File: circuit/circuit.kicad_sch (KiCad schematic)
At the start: 23 parts, among them SW101 SW_Push, SW102 SW_Push, SW103 SW_Push, SW104 SW_Push, SW105 SW_Push, SW106 SW_Push, SW107 SW_Push, SW108 SW_Push, SW109 SW_Push, SW110 SW_Push, U5 ESP32-S3-DevKitC

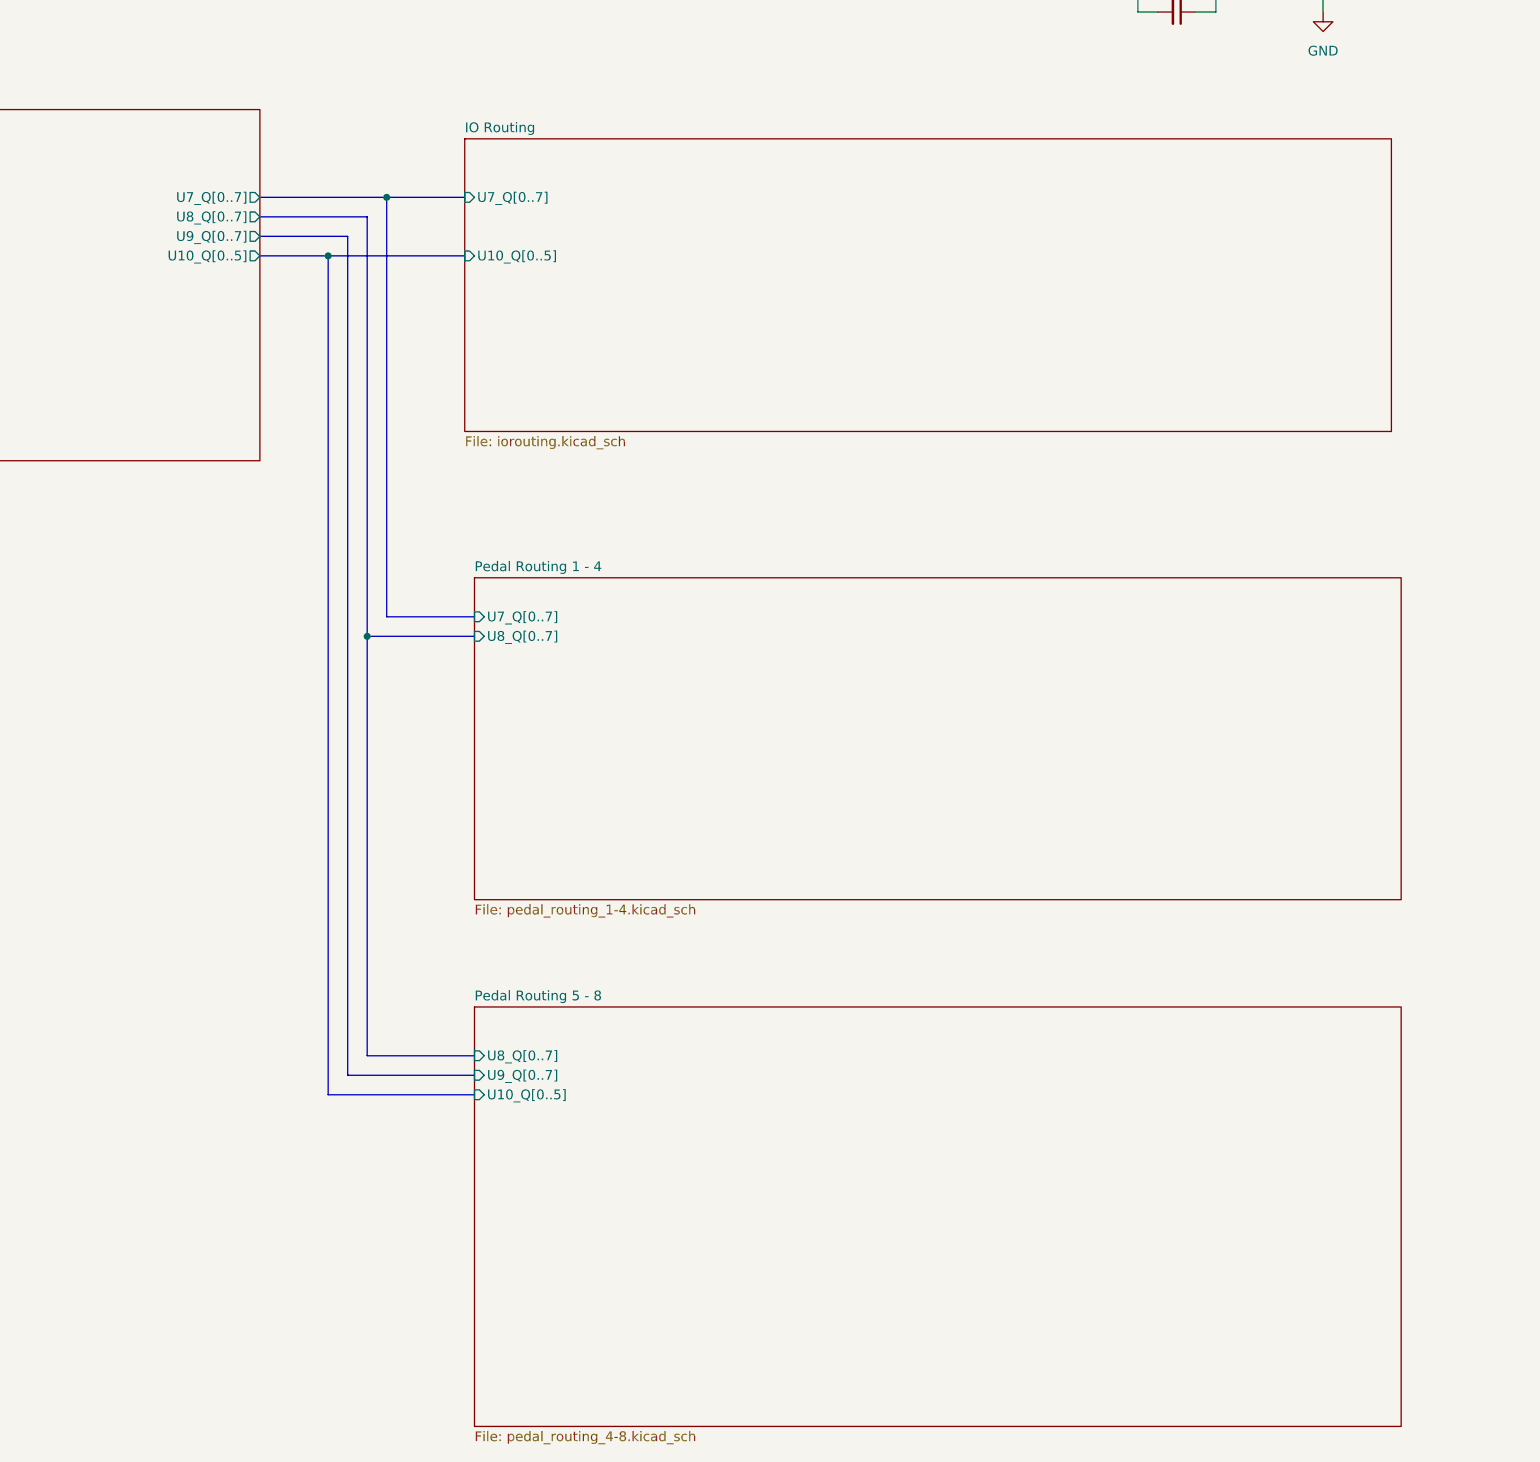
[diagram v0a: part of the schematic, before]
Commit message: Hopefully close to finished
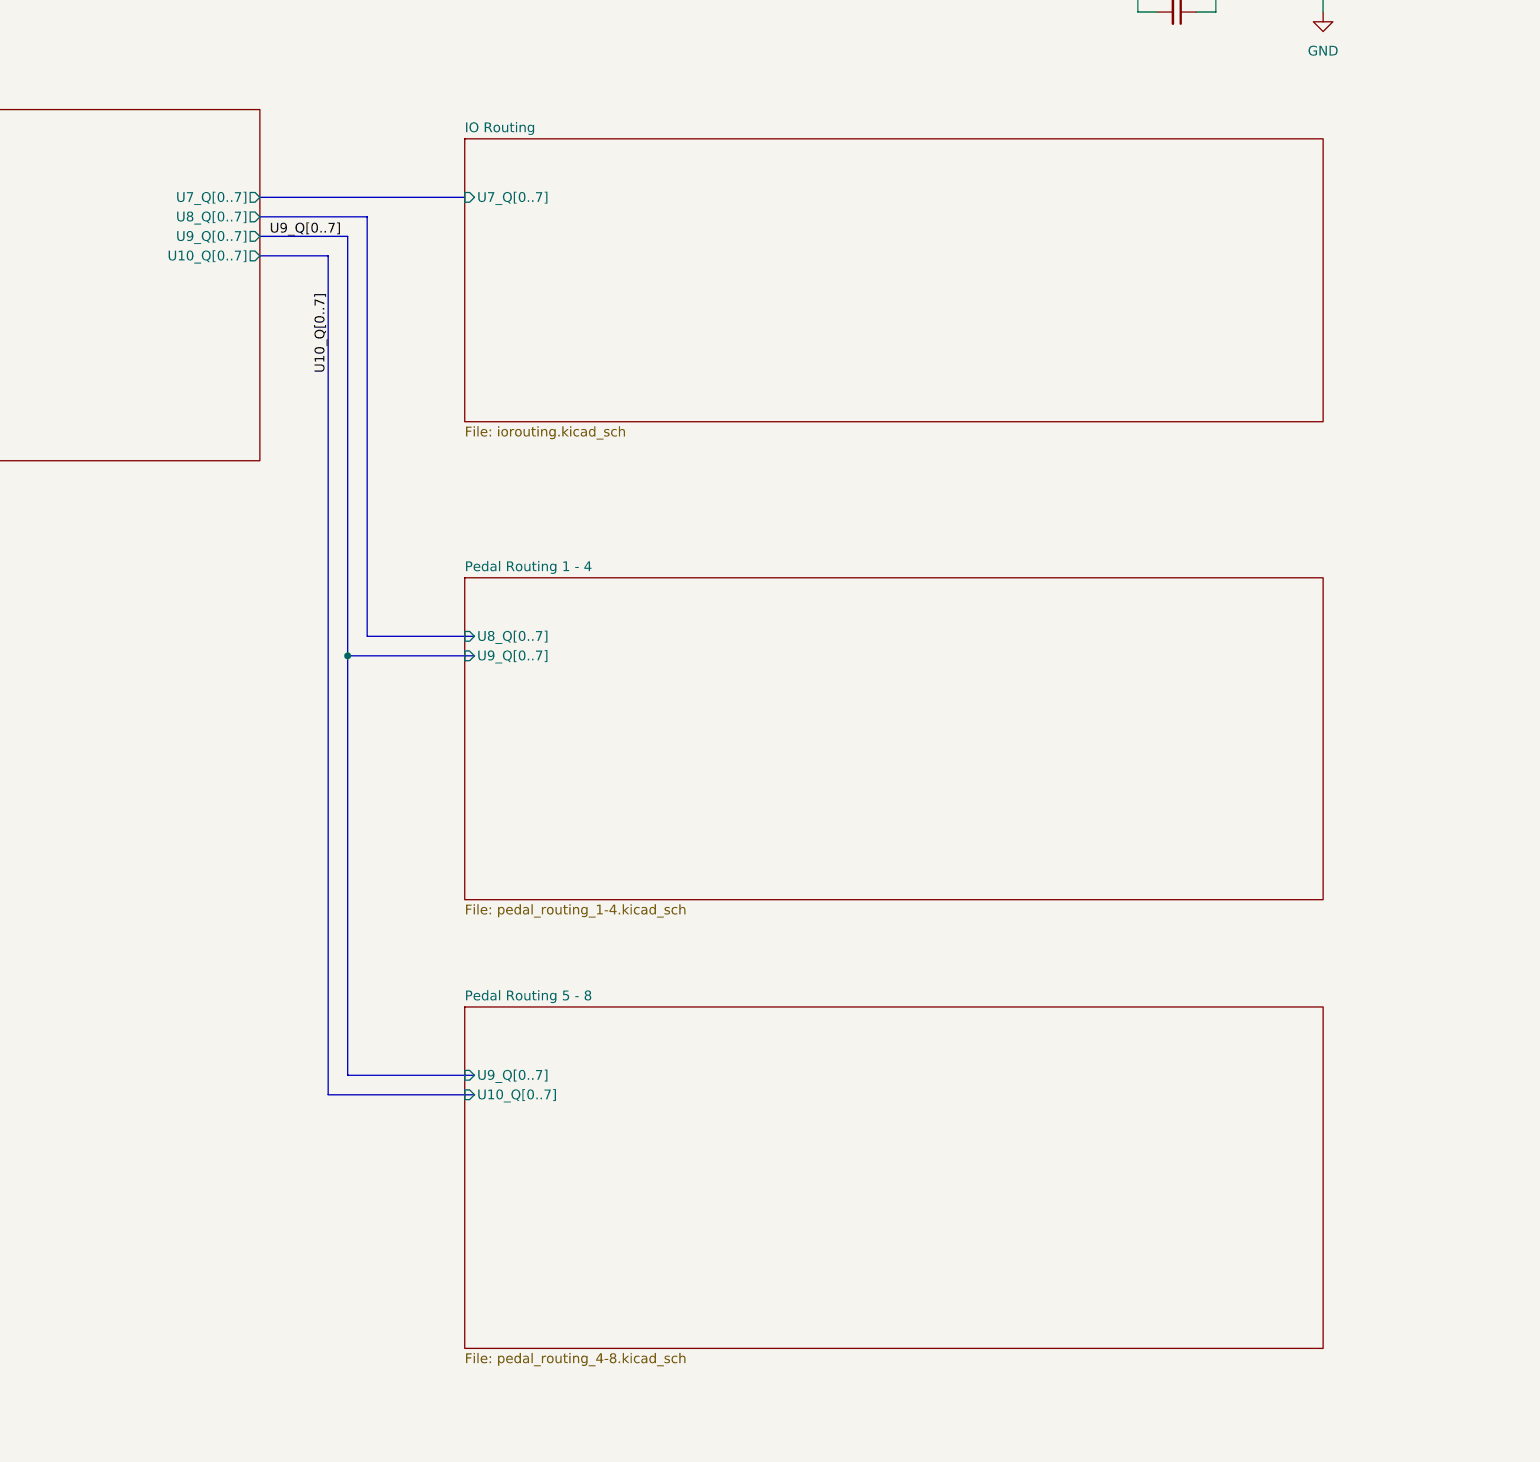
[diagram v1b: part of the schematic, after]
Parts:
- removed U5: ESP32-S3-DevKitC, Esp32 DevKits:ESP32-S3-DevKitC, symbol PCM_Espressif:ESP32-S3-DevKitC
- added U5: ESP32-S3-DevKitC, ESP:ESP32-S3-DevKitC, symbol Espressif:ESP32-S3-DevKitC
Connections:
- net +5V: now also U5.21 (5V)
- net 3.3V: now also U5.1 (3V3), U5.2 (3V3)
- net GND: now also U5.22 (GND), U5.23 (GND), U5.24 (GND), U5.44 (GND)
- net SR_DS: now also U5.9 (GPIO16/ADC2_CH5/32K_N)
- net SR_OE: now also U5.25 (GPIO19/USB_D-)
- net SR_SHCP: now also U5.10 (GPIO17/ADC2_CH6)
- net SR_STCP: now also U5.11 (GPIO18/ADC2_CH7)
- net at C103.2, SW103.1: now also U5.12 (GPIO8/ADC1_CH7)
- net at C105.2, SW105.1: now also U5.16 (GPIO10/ADC1_CH9)
- net at C107.2, SW107.1: now also U5.18 (GPIO12/ADC2_CH1)
- net at Disp101.2 (SDA): now also U5.4 (GPIO4/ADC1_CH3)
- net at Disp101.3 (SCL): now also U5.5 (GPIO5/ADC1_CH4)
- net at C106.2, SW106.1: now also U5.17 (GPIO11/ADC2_CH0)
- net at C109.2, SW109.1: now also U5.20 (GPIO14/ADC2_CH3)
- net at C102.2, SW102.1: now also U5.7 (GPIO7/ADC1_CH6)
- net at C108.2, SW108.1: now also U5.19 (GPIO13/ADC2_CH2)
- net at C110.2, SW110.1: now also U5.8 (GPIO15/ADC2_CH4/32K_P)
- net at C104.2, SW104.1: now also U5.15 (GPIO9/ADC1_CH8)
- net at C101.2, SW101.1: now also U5.6 (GPIO6/ADC1_CH5)
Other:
- sheet IO Routing ports: added none; removed U10_Q[0..5]
- sheet Pedal Routing 1 - 4 ports: added U9_Q[0..7]; removed U7_Q[0..7]
- sheet Pedal Routing 5 - 8 ports: added U10_Q[0..7]; removed U10_Q[0..5], U8_Q[0..7]
- sheet Shift Registers ports: added U10_Q[0..7]; removed U10_Q[0..5]
